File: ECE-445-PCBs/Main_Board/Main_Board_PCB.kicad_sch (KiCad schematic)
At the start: 5 parts, among them J1 USB_C_Receptacle_USB2.0_16P, J2 Screw_Terminal_01x08, J3 Conn_01x02_Pin, U1 ESP32-S3-WROOM-1, U2 TLV62569DDC

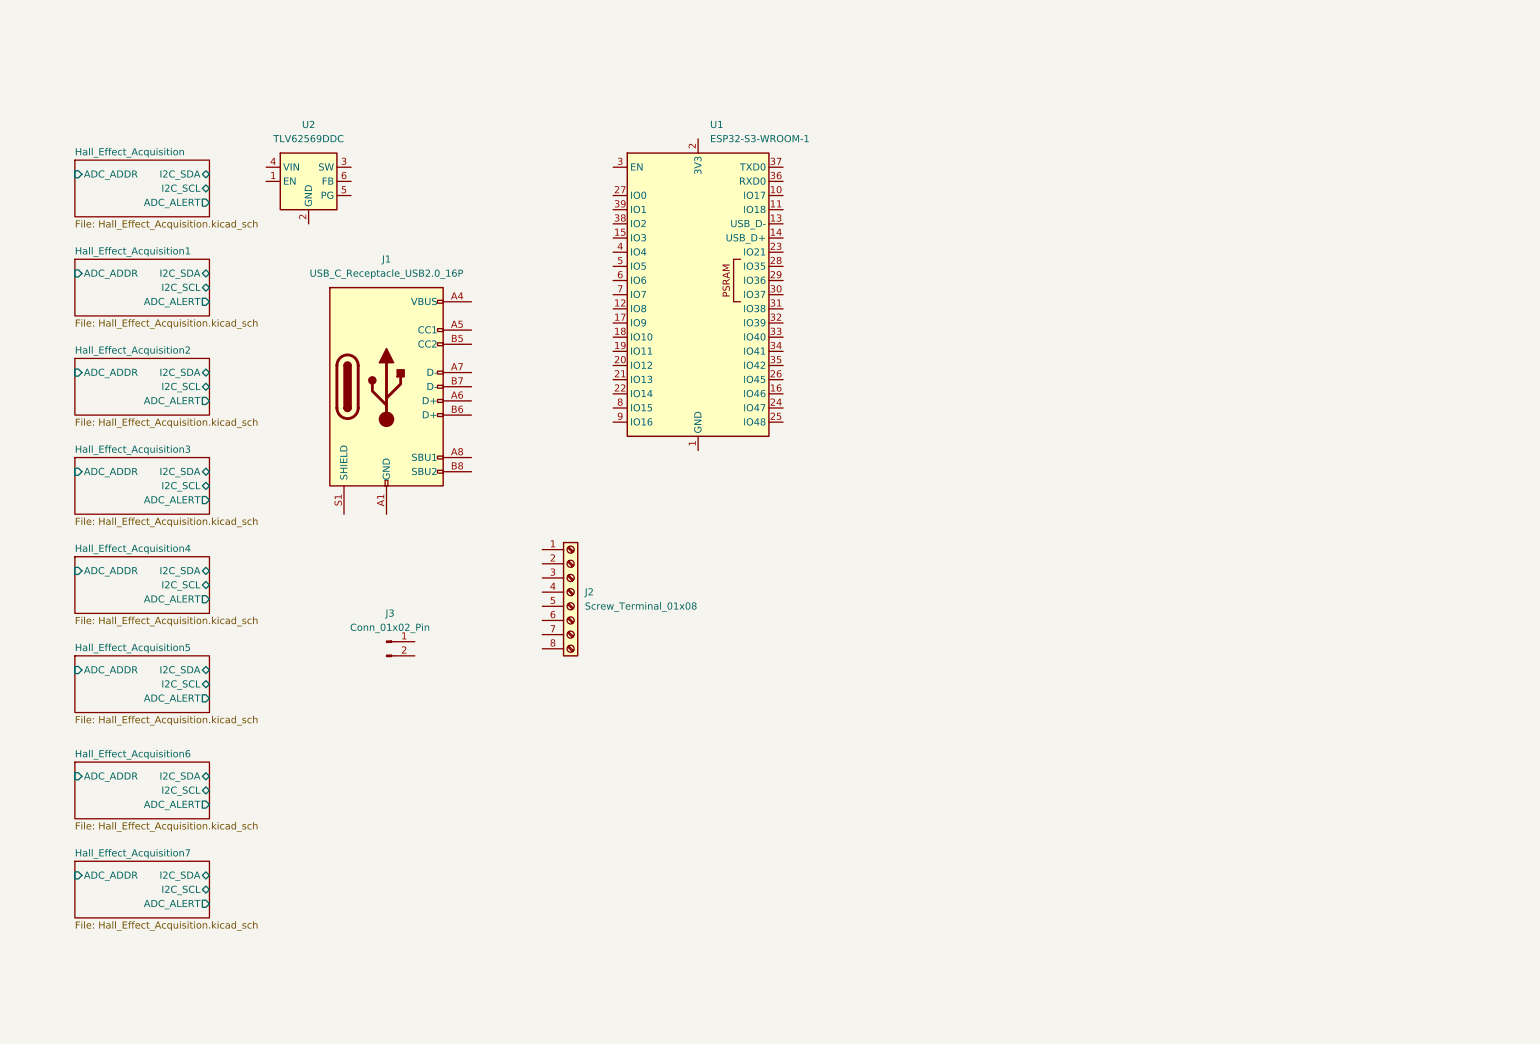
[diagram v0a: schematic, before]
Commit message: PSU done
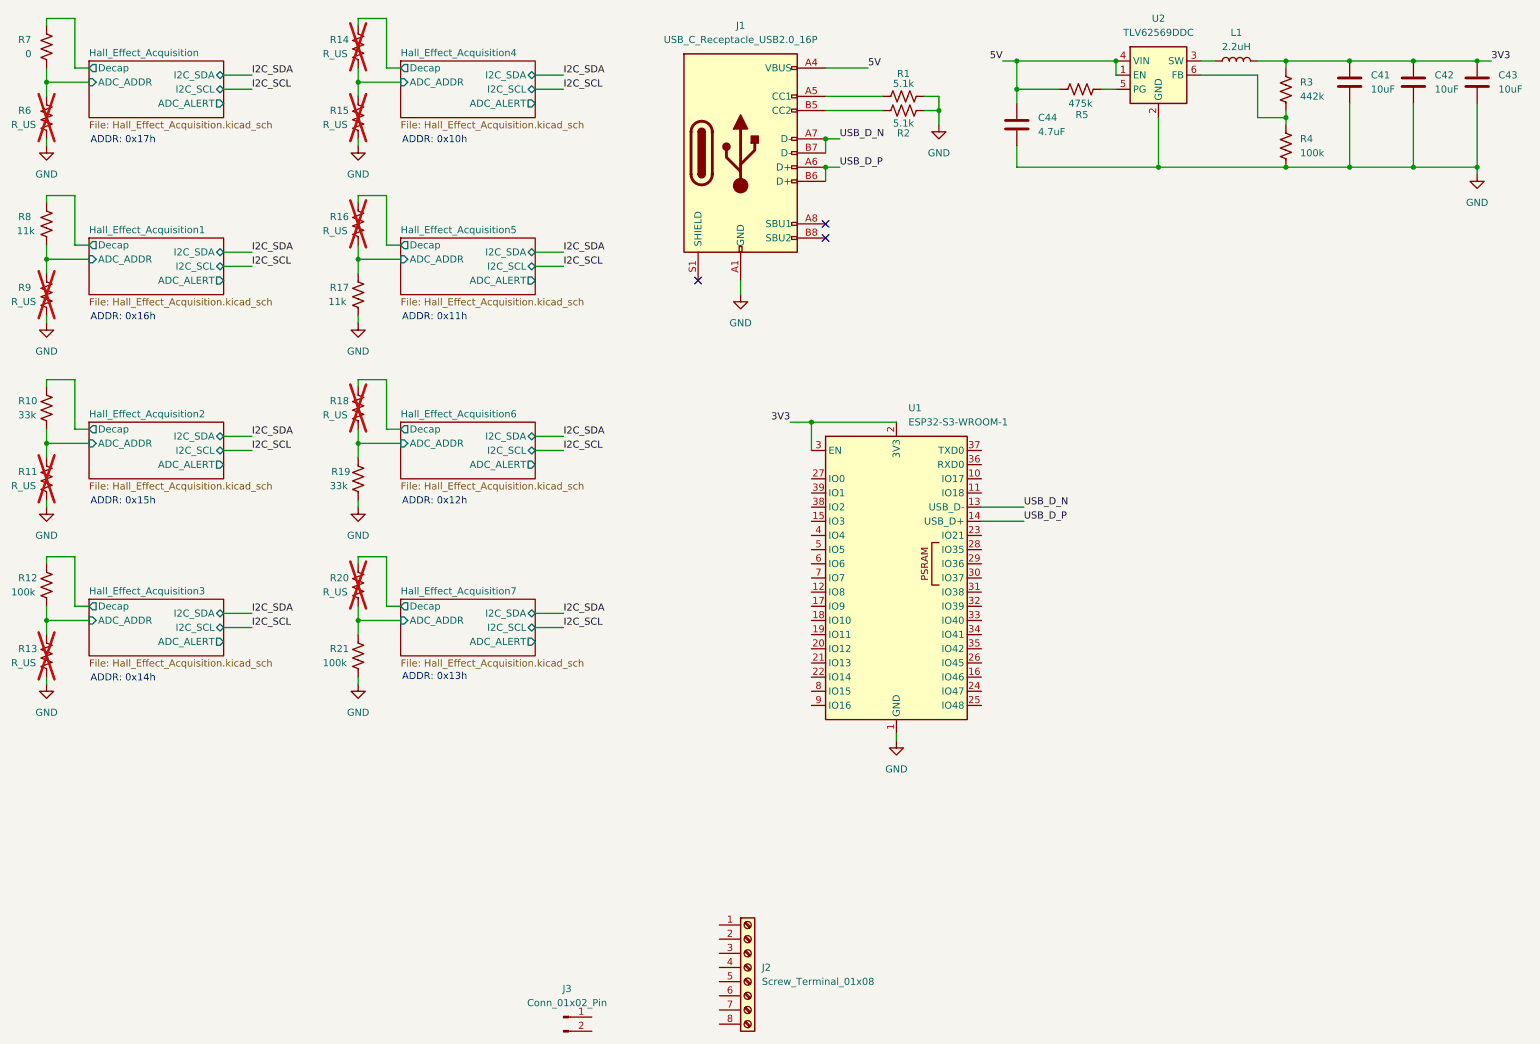
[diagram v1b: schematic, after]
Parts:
- added C41, C42, C43: 10uF, symbol Device:C
- added C44: 4.7uF, symbol Device:C
- added L1: 2.2uH, symbol Device:L
- added R1, R2: 5.1k, symbol Device:R_US
- added R10, R19: 33k, symbol Device:R_US
- added R11, R13, R14, R15, R16, R18, R20, R6, R9: R_US, symbol Device:R_US
- added R12, R21, R4: 100k, symbol Device:R_US
- added R17, R8: 11k, symbol Device:R_US
- added R3: 442k, symbol Device:R_US
- added R5: 475k, symbol Device:R_US
- added R7: 0, symbol Device:R_US
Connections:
- net Hall_Effect_Acquisition/ADC_ADDR: now also R6.1, R7.2
- net Hall_Effect_Acquisition1/ADC_ADDR: now also R8.2, R9.1
- net Hall_Effect_Acquisition2/ADC_ADDR: now also R10.2, R11.1
- net Hall_Effect_Acquisition3/ADC_ADDR: now also R12.2, R13.1
- net Hall_Effect_Acquisition4/ADC_ADDR: now also R14.2, R15.1
- net Hall_Effect_Acquisition5/ADC_ADDR: now also R16.2, R17.1
- net Hall_Effect_Acquisition6/ADC_ADDR: now also R18.2, R19.1
- net Hall_Effect_Acquisition7/ADC_ADDR: now also R20.2, R21.1
- net GND: now reaches U1.1 (GND), U1.40 (GND), U1.41 (GND)
- net GND: now also J1.A1 (GND), J1.A12 (GND), J1.B1 (GND), J1.B12 (GND), U2.2 (GND), C41.1, C42.1, C43.1, C44.1, R1.2, R11.2, R13.2, R15.2, R17.2, R19.2, R2.1, R21.2, R4.2, R6.2, R9.2
- net USB_D_N: now reaches U1.13 (USB_D-)
- net USB_D_N: now also J1.A7 (D-), J1.B7 (D-)
- net USB_D_P: now reaches U1.14 (USB_D+)
- net USB_D_P: now also J1.A6 (D+), J1.B6 (D+)
- net 3V3: now reaches U1.2 (3V3)
- net 3V3: now also U1.3 (EN), C41.2, C42.2, C43.2, L1.2, R3.1
- net 5V: now reaches J1.A4 (VBUS), J1.A9 (VBUS), J1.B4 (VBUS), J1.B9 (VBUS)
- net 5V: now also U2.1 (EN), U2.4 (VIN), C44.2, R5.2
- net at J1.A5 (CC1): now also R1.1
- net at J1.B5 (CC2): now also R2.2
- net at U2.3 (SW): now also L1.1
- net at U2.5 (PG): now also R5.1
- net at U2.6 (FB): now also R3.2, R4.1
- new net Hall_Effect_Acquisition/Decap: R7.1
- new net Hall_Effect_Acquisition1/Decap: R8.1
- new net Hall_Effect_Acquisition2/Decap: R10.1
- new net Hall_Effect_Acquisition3/Decap: R12.1
- new net Hall_Effect_Acquisition4/Decap: R14.1
- new net Hall_Effect_Acquisition5/Decap: R16.1
- new net Hall_Effect_Acquisition6/Decap: R18.1
- new net Hall_Effect_Acquisition7/Decap: R20.1
- no-connect marks 0 -> 3
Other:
- sheet Hall_Effect_Acquisition ports: added Decap; removed none
- sheet Hall_Effect_Acquisition1 ports: added Decap; removed none
- sheet Hall_Effect_Acquisition2 ports: added Decap; removed none
- sheet Hall_Effect_Acquisition3 ports: added Decap; removed none
- sheet Hall_Effect_Acquisition4 ports: added Decap; removed none
- sheet Hall_Effect_Acquisition5 ports: added Decap; removed none
- sheet Hall_Effect_Acquisition6 ports: added Decap; removed none
- sheet Hall_Effect_Acquisition7 ports: added Decap; removed none
- note added: "ADDR: 0x10h"
- note added: "ADDR: 0x11h"
- note added: "ADDR: 0x12h"
- note added: "ADDR: 0x13h"
- note added: "ADDR: 0x14h"
- note added: "ADDR: 0x15h"
- note added: "ADDR: 0x16h"
- note added: "ADDR: 0x17h"
- moved on the sheet: J1, J2, J3, U1, U2
